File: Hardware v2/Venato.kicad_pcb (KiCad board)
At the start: 2 copper layers, 21 x 47 mm, 24 parts, among them J1 Conn_01x02_Male, J2 Conn_01x02_Male, J3 Conn_01x02_Male, J4 Conn_01x02_Male, J5 Conn_01x02_Male, J6 Conn_01x15_Female, J7 Conn_01x15_Female, U1 LM317_TO-220, U2 MCP6002-xP, U3 MCP6002-xP, U4 MCP6002-xP

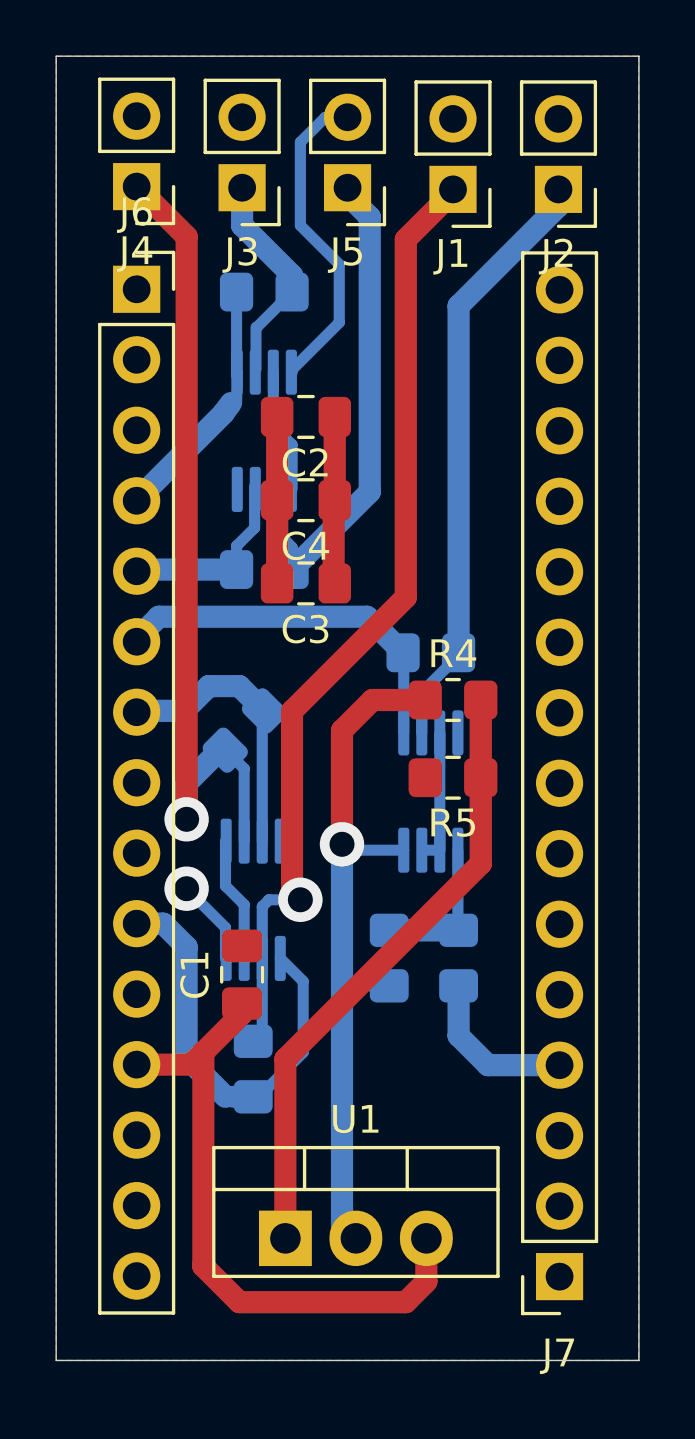
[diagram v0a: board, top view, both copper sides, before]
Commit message: v2 pcb done
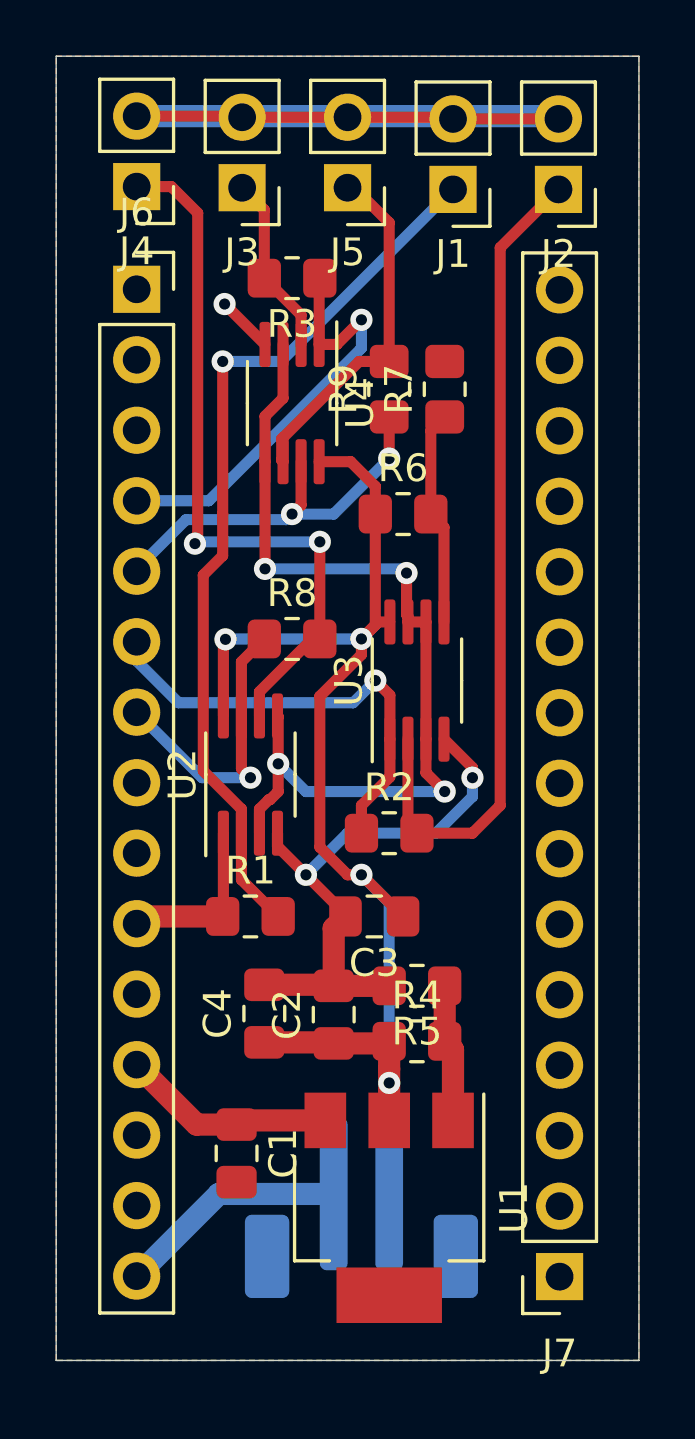
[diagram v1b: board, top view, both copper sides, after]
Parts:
- added J8: Conn_01x02_Male, Connector_JST:JST_PH_B2B-PH-SM4-TB_1x02-1MP_P2.00mm_Vertical, B.Cu at (240.0, 104.5)
- R1, R2, R3, R6, R7, R8, R9, U2, U3, U4: moved to F.Cu
- U1: footprint Package_TO_SOT_THT:TO-220-3_Vertical -> Package_TO_SOT_SMD:SOT-223
- moved C2 21.6 mm to (239.0, 97.5), turned to 90 degrees
- moved R7 20.5 mm to (243.0, 75.0), turned to 90 degrees
- moved C4 18.6 mm to (236.5, 97.5), turned to 90 degrees
- moved R6 16.0 mm to (241.5, 79.5), turned to 0 degrees
- moved R4 12.4 mm to (242.0, 98.5)
- moved C3 12.3 mm to (240.5, 94.0)
- moved R9 7.91 mm to (241.0, 75.0), turned to 90 degrees
- moved R5 7.61 mm to (242.0, 96.5)
- moved R2 6.67 mm to (241.0, 91.0)
- moved C1 6.44 mm to (235.5, 102.5), turned to 270 degrees
- moved R1 5.50 mm to (236.0, 94.0), turned to 0 degrees
- moved U2 4.51 mm to (236.0, 88.9)
- moved U3 4.03 mm to (242.0, 85.5), turned to 90 degrees
- moved U1 3.90 mm to (241.0, 104.5), turned to 270 degrees
- moved R8 3.71 mm to (237.5, 84.0), turned to 0 degrees
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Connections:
- J6 pad 15: (no net) -> VIN
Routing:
- net GND: track 26.6 -> 53.5 mm, vias 1 -> 3
- net VGND: track 13.8 -> 33.3 mm, vias 0 -> 4
- net Net-(R4-Pad2): track 22.3 -> 4.97 mm
- net +5V: track 23.0 -> 7.76 mm
- net +3.3VA: track 32.1 -> 44.5 mm, vias 1 -> 4
- net SENSE1: track 14.9 -> 6.22 mm
- net Net-(J2-Pad1): track 21.5 -> 30.0 mm
- net VIN: track 0.00 -> 8.33 mm
- net SENSE3: track 6.87 -> 14.3 mm, vias 0 -> 2
- net SENSE4: track 9.00 -> 15.7 mm, vias 0 -> 1
- net Net-(J5-Pad1): track 18.1 -> 13.8 mm
- net Net-(J4-Pad1): track 30.1 -> 26.4 mm, vias 1 -> 2
- net SENSE2: track 13.4 -> 16.4 mm, vias 0 -> 1
- net Net-(R6-Pad2): track 5.40 -> 7.79 mm
- net Net-(J1-Pad1): track 34.6 -> 32.3 mm
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- added copper zone on B.Cu, net GND
